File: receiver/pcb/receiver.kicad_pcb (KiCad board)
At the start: 4 copper layers, 41 x 41 mm, 27 parts, among them IC1 L7806CD2T-TR, U1 XIAO ESP32C3

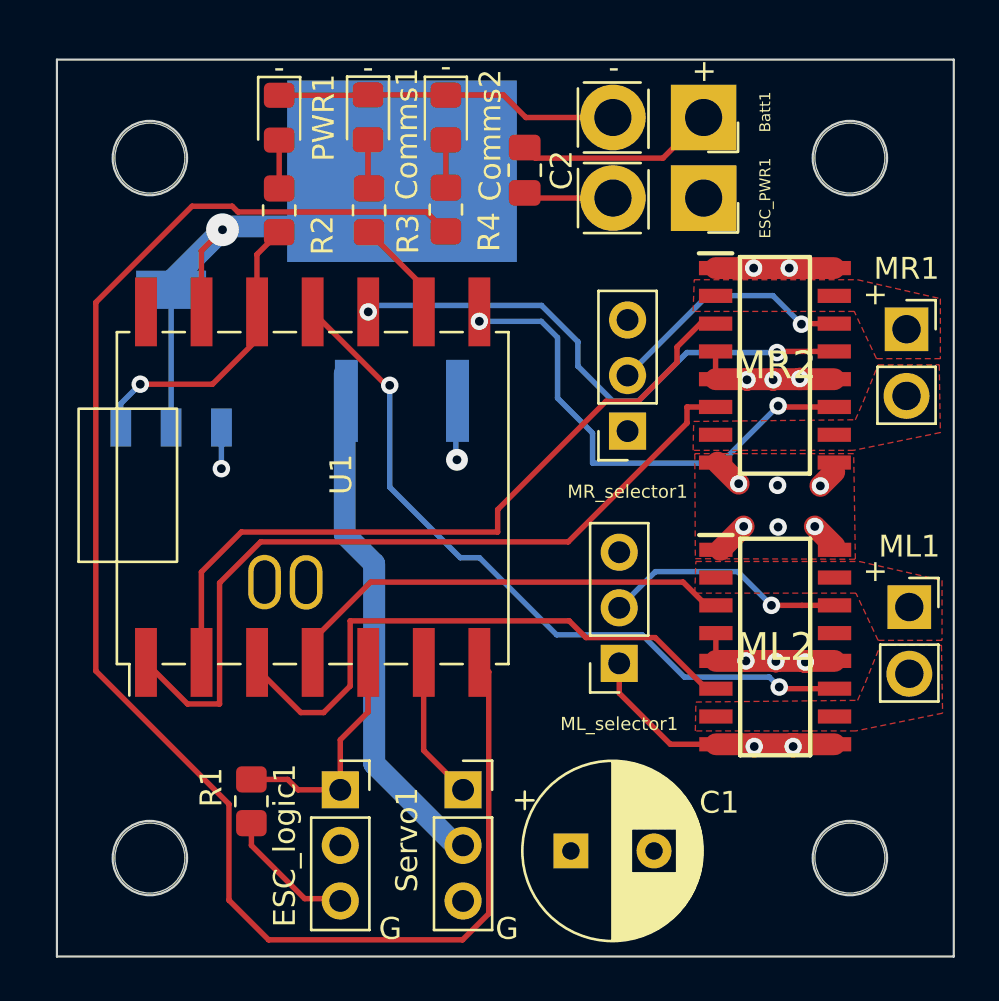
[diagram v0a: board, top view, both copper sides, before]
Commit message: V9 ready to order
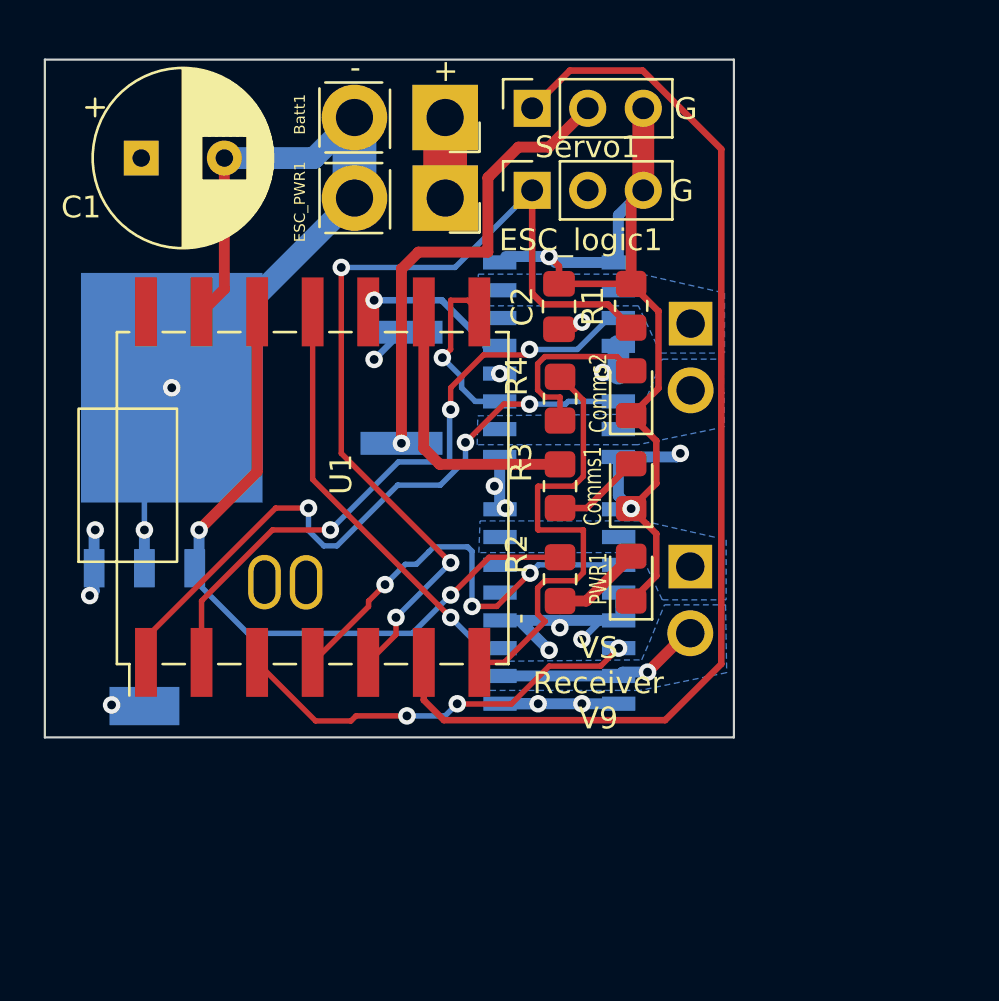
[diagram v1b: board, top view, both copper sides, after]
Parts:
- removed H1, H2, H3, H4: MountingHole, MountingHole:MountingHole_3.2mm_M3
- removed ML_selector1: ML_selector, Connector_PinSocket_2.54mm:PinSocket_1x03_P2.54mm_Vertical
- removed MR_selector1: MR_selector, Connector_PinSocket_2.54mm:PinSocket_1x03_P2.54mm_Vertical
- ML1, ML2, MR1, MR2: moved to B.Cu
- moved C1 37.3 mm to (150.4, 83.0)
- moved Servo1 31.3 mm to (168.2, 80.7), turned to 90 degrees
- moved ESC_logic1 28.8 mm to (168.2, 84.5), turned to 90 degrees
- moved R1 28.5 mm to (172.8, 89.8), turned to -90 degrees
- moved PWR1 26.5 mm to (172.8, 102.2), turned to 90 degrees
- moved R2 21.2 mm to (169.5, 102.2), turned to -90 degrees
- moved Comms1 20.7 mm to (172.8, 98.0), turned to 90 degrees
- moved R3 15.3 mm to (169.5, 98.0), turned to -90 degrees
- moved Comms2 15.2 mm to (172.8, 93.8), turned to 90 degrees
- moved PS1 12.8 mm to (150.5, 104.9), turned to -90 degrees
- moved Batt1 11.8 mm to (163.0, 81.1)
- moved ESC_PWR1 11.8 mm to (163.0, 84.8)
- moved ML1 10.2 mm to (175.5, 101.7), turned to 180 degrees
- moved R4 10.1 mm to (169.5, 94.0), turned to -90 degrees
- moved ML2 10.0 mm to (169.5, 103.5), turned to 180 degrees
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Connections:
- ML2 pad 14: Net-(ML2-SEL0) -> unconnected-(ML2-SEL0-Pad14)
- MR2 pad 14: Net-(MR2-SEL0) -> unconnected-(MR2-SEL0-Pad14)
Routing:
- net Net-(U1-D6): track 72.9 -> 21.5 mm
- net Net-(Servo1-Pin_1): track 6.59 -> 51.2 mm
- net Net-(ESC_logic1-Pin_1): track 10.6 -> 41.8 mm, vias 0 -> 3
- net GND: track 74.6 -> 96.3 mm, vias 11 -> 10
- net +3V3: track 13.9 -> 32.6 mm, vias 1 -> 2
- net /MR_sense: track 25.6 -> 7.25 mm, vias 2 -> 1
- net /MR_PWM: track 22.4 -> 8.05 mm, vias 2 -> 1
- net /ML_PWM: track 33.7 -> 19.4 mm, vias 2 -> 1
- net Net-(MR2-SEL0): track 11.5 -> 0.00 mm, vias 1 -> 0
- net Net-(ML2-SEL0): track 11.2 -> 0.00 mm, vias 1 -> 0
- net Net-(ML1-Pin_2): track 0.04 -> 9.51 mm, vias 0 -> 1
- net Net-(U1-D8): track 4.66 -> 12.8 mm
- net Net-(ML2-INB): track 26.9 -> 19.0 mm, vias 0 -> 3
- net Net-(MR2-INB): track 36.1 -> 29.7 mm, vias 0 -> 3
- net Net-(Comms2-A): track 2.18 -> 8.11 mm
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- added copper zone on B.Cu, net Net-(ML1-Pin_1)
- added copper zone on B.Cu, net Net-(ML1-Pin_2)
- added copper zone on B.Cu, net Net-(MR1-Pin_1)
- added copper zone on B.Cu, net Net-(MR1-Pin_2)
- removed copper zone on F.Cu, net GND
- removed copper zone on F.Cu, net Net-(ML1-Pin_1)
- removed copper zone on F.Cu, net Net-(ML1-Pin_2)
- removed copper zone on F.Cu, net Net-(MR1-Pin_1)
- removed copper zone on F.Cu, net Net-(MR1-Pin_2)
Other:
- board size 41 x 41 mm -> 31.5 x 31 mm
- board text added: "VS Receiver V9"
- board text removed: "32x32mm mounting holes"
- board text removed: "VS Receiver V8"
